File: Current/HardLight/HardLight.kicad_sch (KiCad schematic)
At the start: 45 parts, among them J0 USB, J1 qwiic, U0 RP2040, U1 LDO-3.3, U2 USBLC6-2SC6, U3 W25Q128JVS, Y0 12MHz

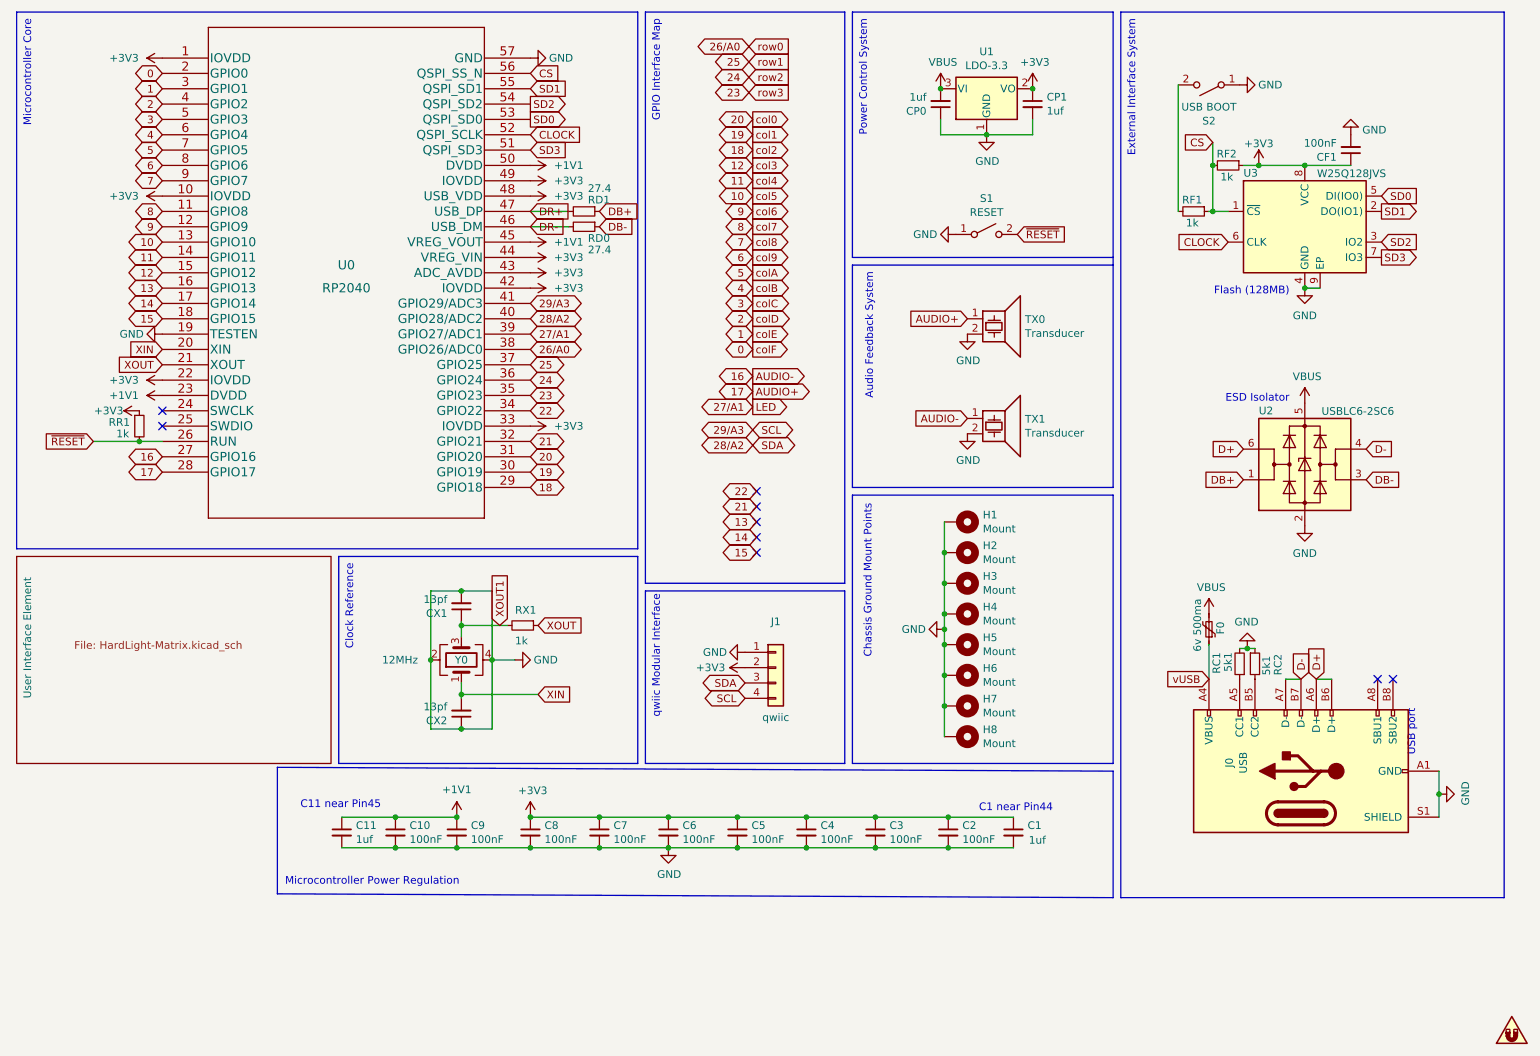
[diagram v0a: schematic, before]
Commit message: eat shit and die
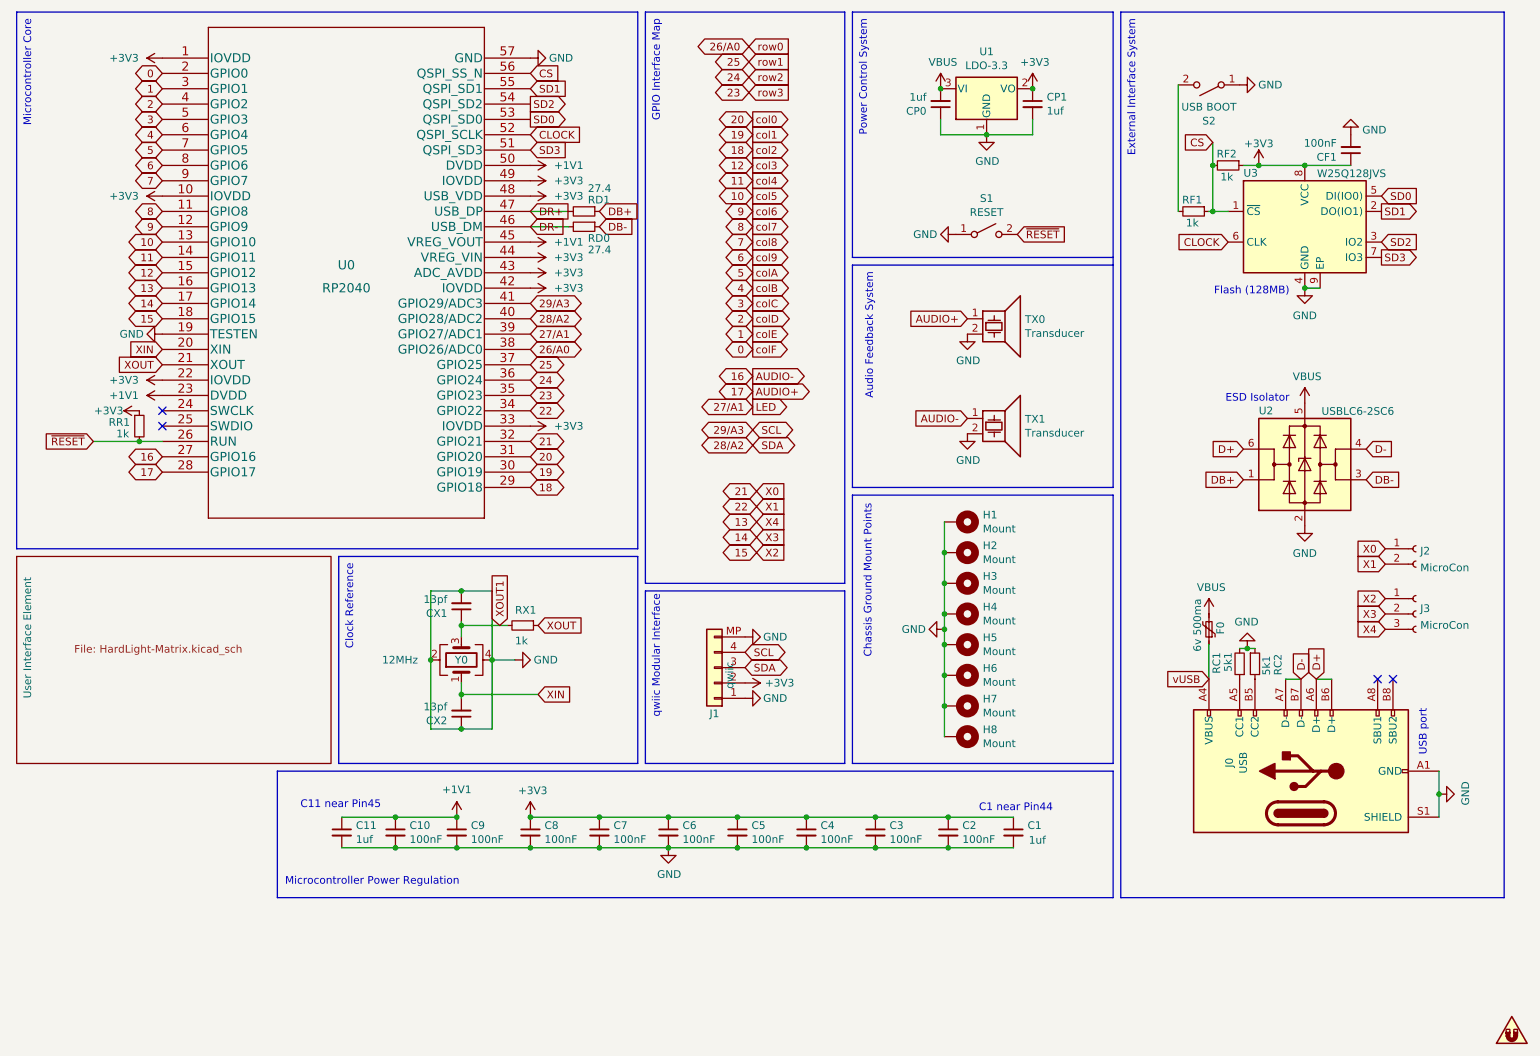
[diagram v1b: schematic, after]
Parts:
- added J2: MicroCon, EDI:MicroCon-2, symbol Connector:Conn_01x02_Female
- added J3: MicroCon, EDI:MicroCon-3, symbol Connector:Conn_01x03_Female
- F0: footprint Fuse:Fuse_0603_1608Metric_Castellated -> Fuse:Fuse_0603_1608Metric
- J1: symbol Connector_Generic:Conn_01x04 -> Connector_Generic:Conn_01x05
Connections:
- net 13: now also J3.3 (Pin_3)
- net 14: now also J3.2 (Pin_2)
- net 15: now also J3.1 (Pin_1)
- net 21: now also J2.1 (Pin_1)
- net 22: now also J2.2 (Pin_2)
- net GND: now also J1.MP
- no-connect marks 9 -> 4
